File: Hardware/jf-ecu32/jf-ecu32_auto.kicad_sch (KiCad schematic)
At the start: 72 parts, among them J1 GAZ, J10 k, J11 RPM, J12 S.PORT, J13 PPM/PWM, J14 PUMP1, J15 PUMP1, J16 PPM/PWM, J17 PUMP2, J18 PUMP2, J19 UART0, J2 AUX, J3 PPM/PWM, J4 STARTER, J5 GLOW, J6 VANNE KEROSTART, J7 VANNE KERO, J8 BATTERY 2S/3S, J9 STARTER, Q1 AO3400A, Q2 QM6006D, Q3 AO3400A, Q4 QM6006D, Q5 QM6006D, Q6 QM6006D, U1 ESP32-WROOM-32D, U2 4050, U3 MAX31855KASA, U4 AMS1117-3.3, U5 4050

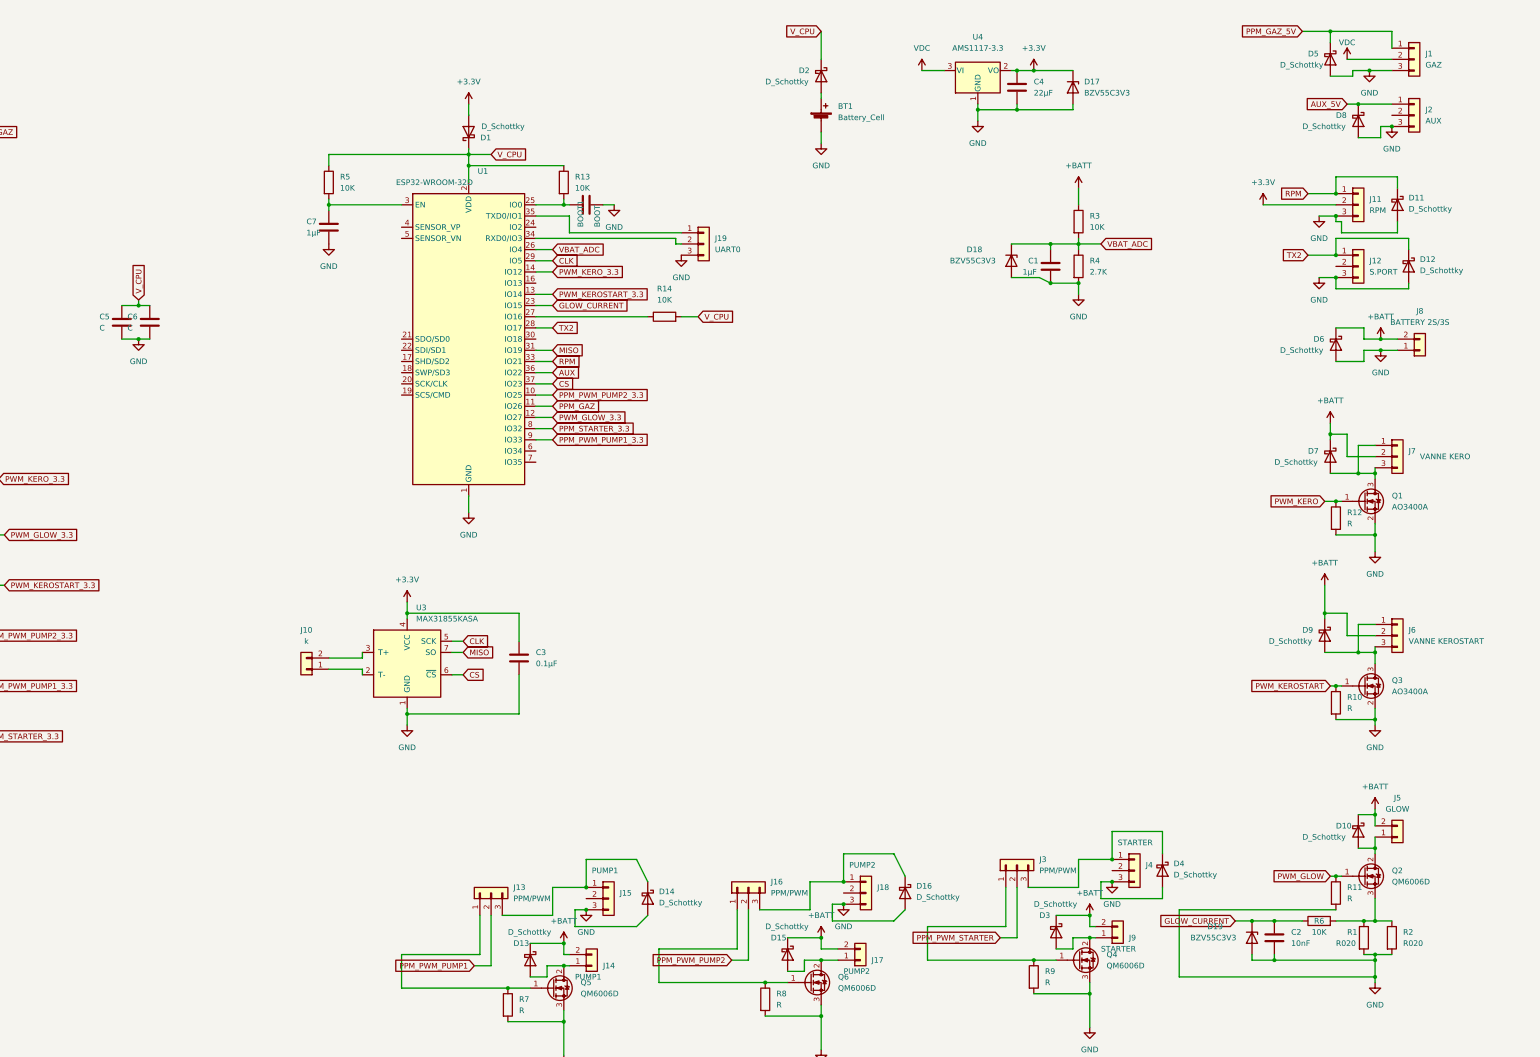
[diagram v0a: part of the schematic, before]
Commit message: pcb
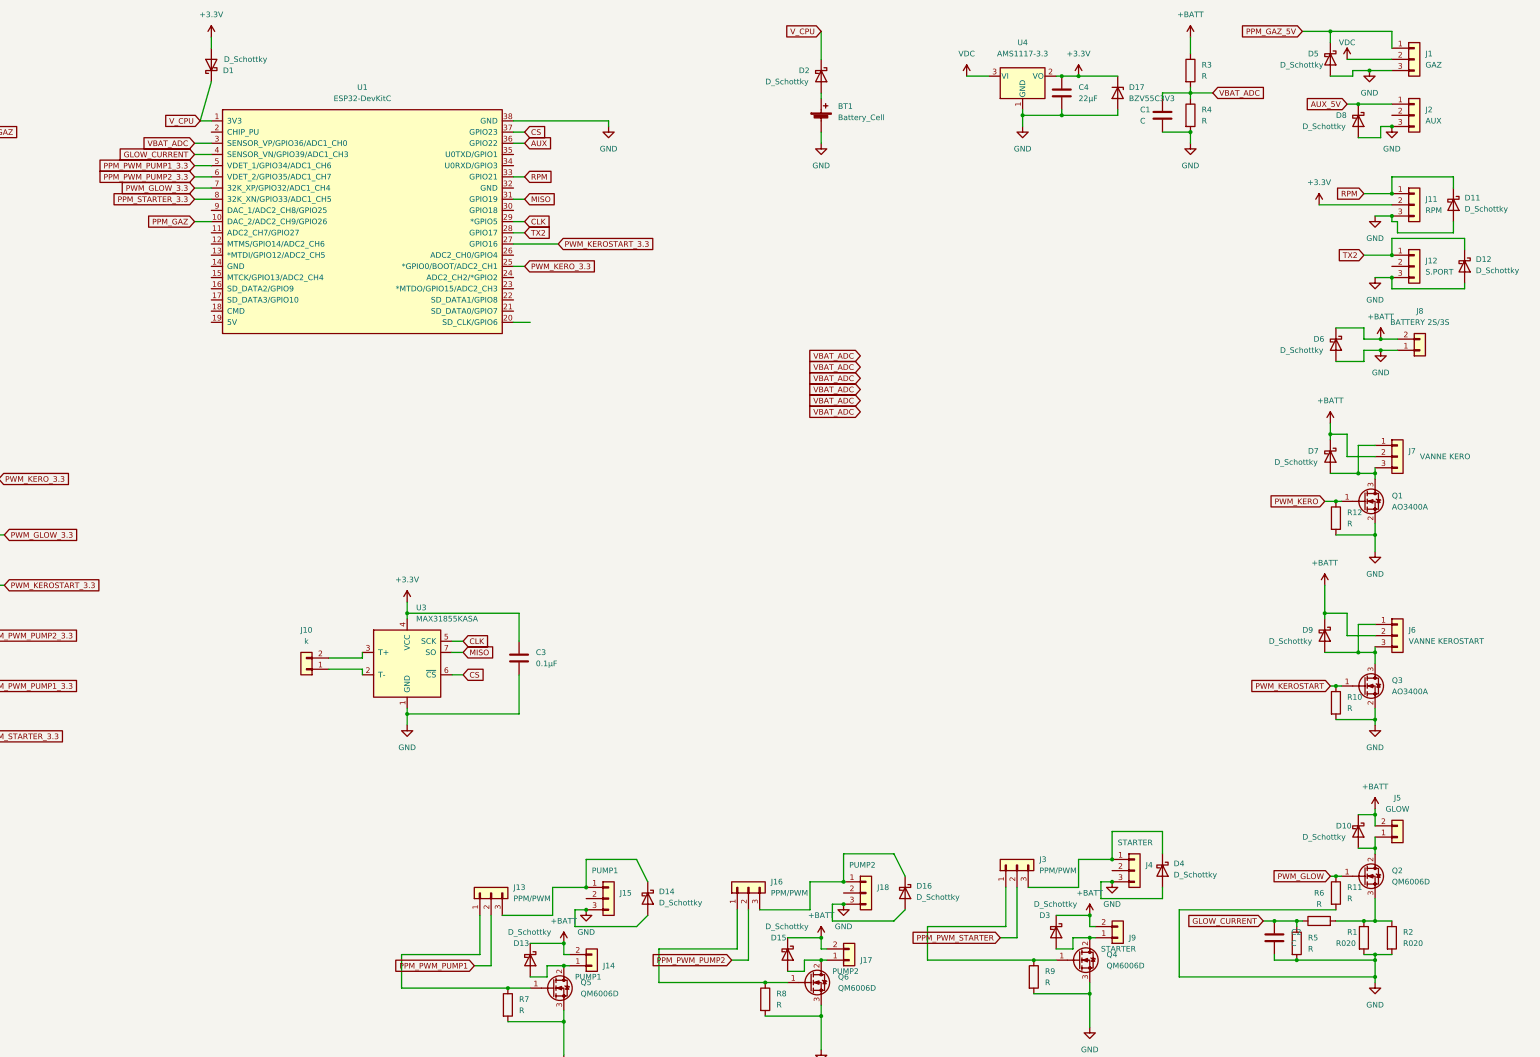
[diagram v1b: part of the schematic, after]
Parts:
- removed BOOT1: BOOT, Capacitor_SMD:C_0603_1608Metric, symbol Device:C
- removed C5, C6: C, Capacitor_SMD:C_0603_1608Metric, symbol Device:C
- removed C7: 1µF, Capacitor_SMD:C_0603_1608Metric, symbol Device:C
- removed D18, D19: BZV55C3V3, Diode_SMD:D_MiniMELF, symbol Diode:BZV55C3V3
- removed J19: UART0, Connector_PinHeader_2.54mm:PinHeader_1x03_P2.54mm_Vertical, symbol Connector_Generic:Conn_01x03
- removed R13, R14: 10K, Resistor_SMD:R_0603_1608Metric, symbol Device:R
- removed U1: ESP32-WROOM-32D, RF_Module:ESP32-WROOM-32, symbol RF_Module:ESP32-WROOM-32D
- added U1: ESP32-DevKitC, RF_Module:ESP32-WROOM-32, symbol Espressif:ESP32-DevKitC
- C1: value 1µF -> C
- C2: value 10nF -> C
- R3, R5, R6: value 10K -> R
- R4: value 2.7K -> R
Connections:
- net AUX: now also U1.36 (GPIO22)
- net CLK: now also U1.29 (*GPIO5)
- net CS: now also U1.37 (GPIO23)
- net GLOW_CURRENT: now also R5.1, U1.4 (SENSOR_VN/GPIO39/ADC1_CH3)
- net GND: now also R5.2, U1.38 (GND)
- net MISO: now also U1.31 (GPIO19)
- net PPM_GAZ: now also U1.10 (DAC_2/ADC2_CH9/GPIO26)
- net PPM_PWM_PUMP1_3.3: now also U1.5 (VDET_1/GPIO34/ADC1_CH6)
- net PPM_PWM_PUMP2_3.3: now also U1.6 (VDET_2/GPIO35/ADC1_CH7)
- net PPM_STARTER_3.3: now also U1.8 (32K_XN/GPIO33/ADC1_CH5)
- net PWM_GLOW_3.3: now also U1.7 (32K_XP/GPIO32/ADC1_CH4)
- net PWM_KEROSTART_3.3: now also U1.27 (GPIO16)
- net PWM_KERO_3.3: now also U1.25 (*GPIO0/BOOT/ADC2_CH1)
- net RPM: now also U1.33 (GPIO21)
- net TX2: now also U1.28 (GPIO17)
- net VBAT_ADC: now also U1.3 (SENSOR_VP/GPIO36/ADC1_CH0)
- net V_CPU: now also U1.1 (3V3); no longer R5.1
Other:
- moved on the sheet: C1, C4, D1, D11, D12, D17, J11, J12, J17, R3, R4, U4
